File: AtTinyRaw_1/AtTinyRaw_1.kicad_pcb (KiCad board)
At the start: 2 copper layers, 28.2 x 18.3 mm, 12 parts, among them J1 Power, J2 PinOut, J3 USB_B_Micro, U1 ATtiny85-20S, U2 L7805

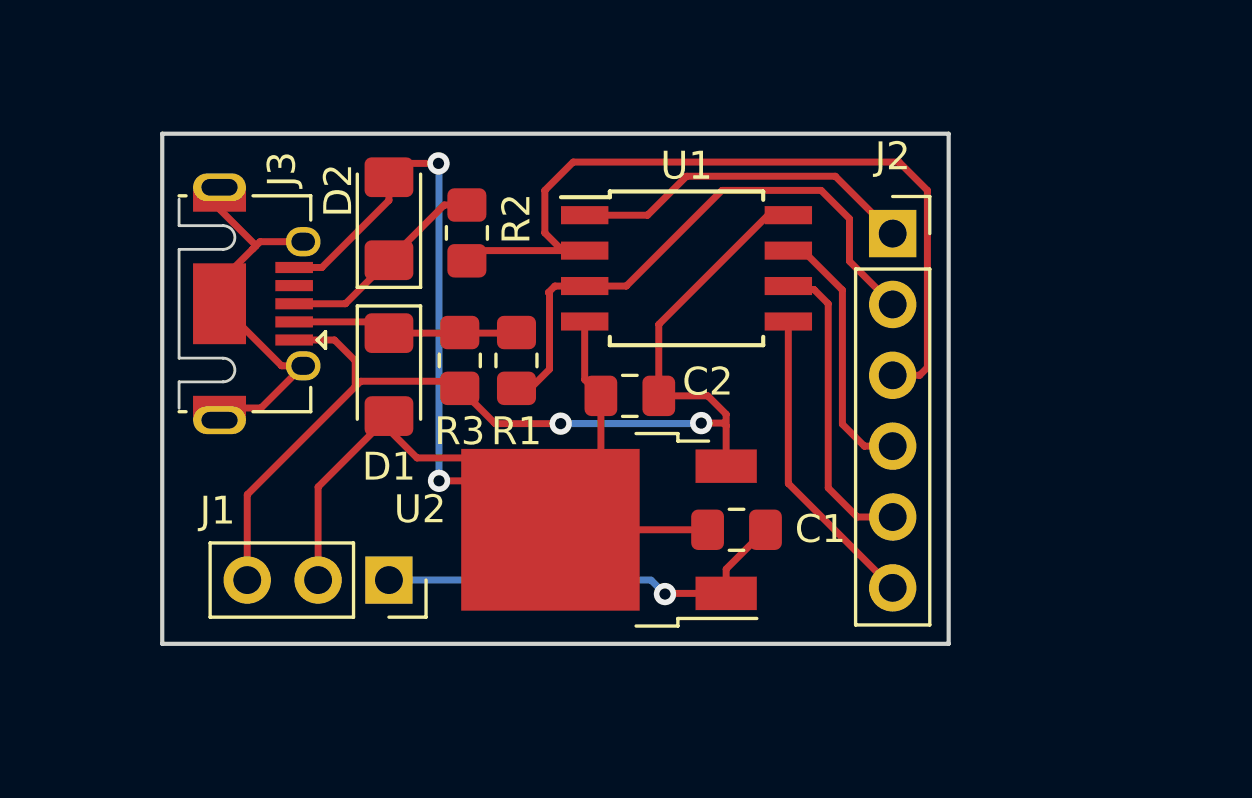
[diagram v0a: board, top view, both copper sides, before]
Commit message: Update
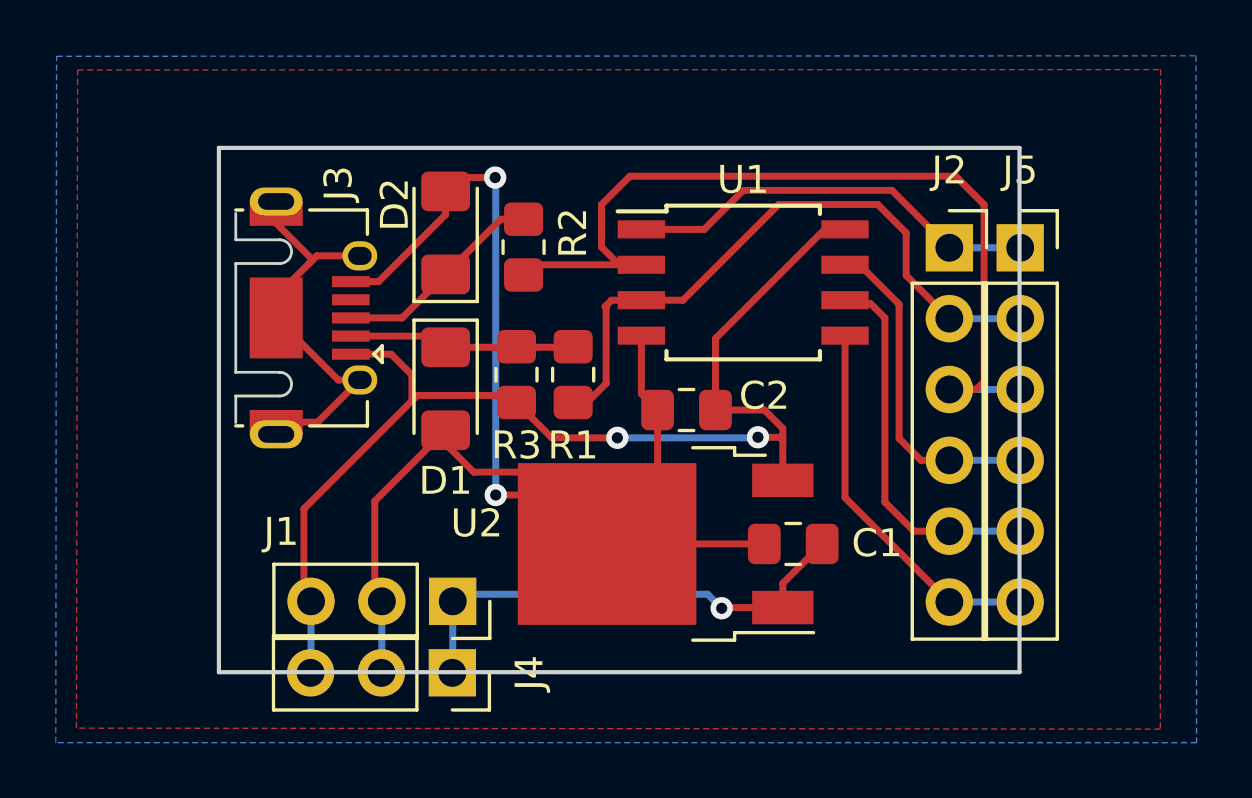
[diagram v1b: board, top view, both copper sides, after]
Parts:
- added J4: Power, Connector_PinSocket_2.54mm:PinSocket_1x03_P2.54mm_Vertical, F.Cu at (180.3, 129.6)
- added J5: PinOut, Connector_PinSocket_2.54mm:PinSocket_1x06_P2.54mm_Vertical, F.Cu at (200.7, 114.3)
- moved J1 2.41 mm to (180.3, 127.0)
- moved J2 2.09 mm to (198.1, 114.3)
- moved J3 2.09 mm to (174.0, 116.8)
- moved C1 2.09 mm to (192.5, 124.9)
- moved C2 2.09 mm to (188.7, 120.1)
- moved D1 2.09 mm to (180.1, 119.4)
- moved D2 2.09 mm to (180.1, 113.8)
- moved R3 2.09 mm to (182.6, 118.9)
- moved R1 2.09 mm to (184.7, 118.9)
- moved R2 2.09 mm to (182.9, 114.3)
- moved U1 2.09 mm to (190.8, 115.6)
- moved U2 2.09 mm to (188.0, 124.9)
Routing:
- net GND: track 53.3 -> 56.0 mm
- net +5V: track 39.4 -> 42.1 mm
- net /PB4: track 20.7 -> 23.0 mm
- net /PB2: track 9.46 -> 11.8 mm
- net /PB0: track 11.1 -> 13.4 mm
- net /PB5: track 12.5 -> 14.8 mm
- net /PB1: track 11.0 -> 13.4 mm
- net /PB3: track 29.9 -> 32.2 mm
- net +VDC: track 15.2 -> 17.4 mm
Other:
- board size 28.2 x 18.3 mm -> 28.7 x 18.8 mm
